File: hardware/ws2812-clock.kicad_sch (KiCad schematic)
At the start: 31 parts, among them J1 Conn_01x01_Pin, Q3 2N7002, SW2 Reset ESP, SW5 Toggle AP, SW6 Toggle Alarm, SW7 Snooze Alarm, U1 ESP32-WROOM-32D, U3 SHT30-DIS, U4 AMS1117-3.3, U5 DMP3026SFDE-7

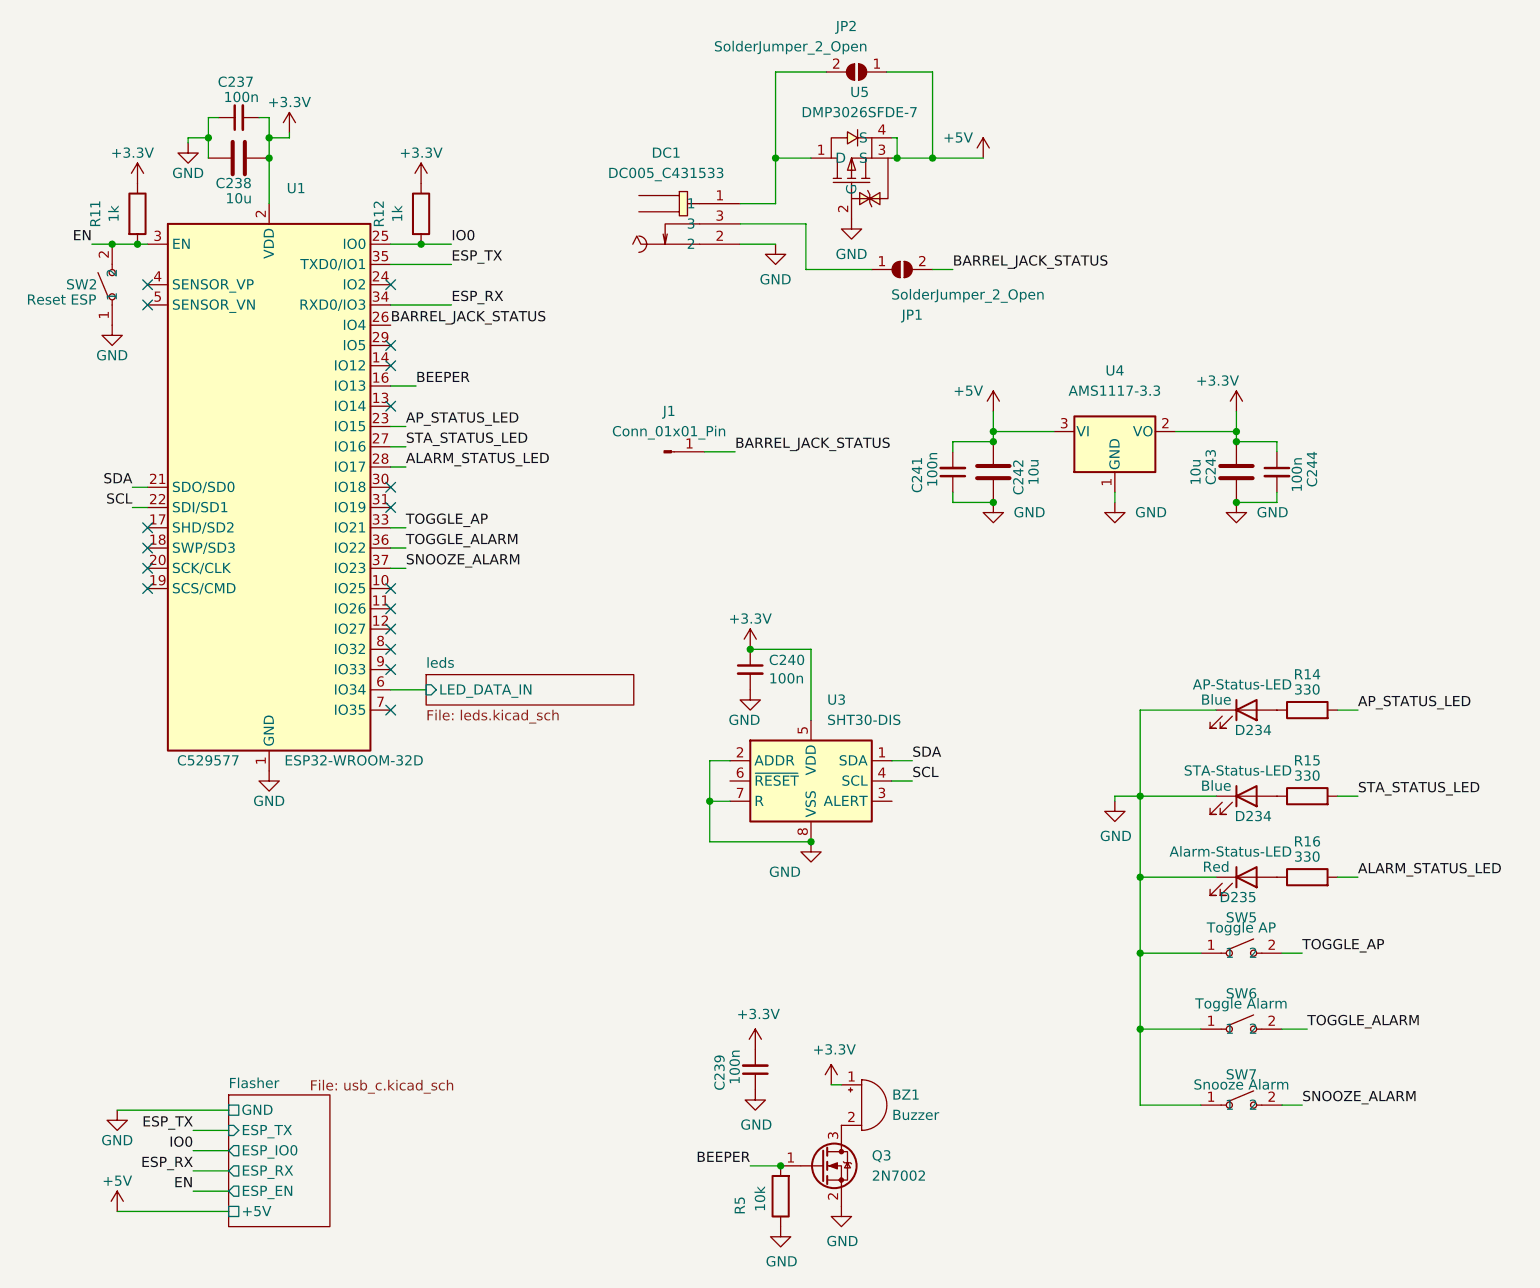
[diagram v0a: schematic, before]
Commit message: Updated PCB
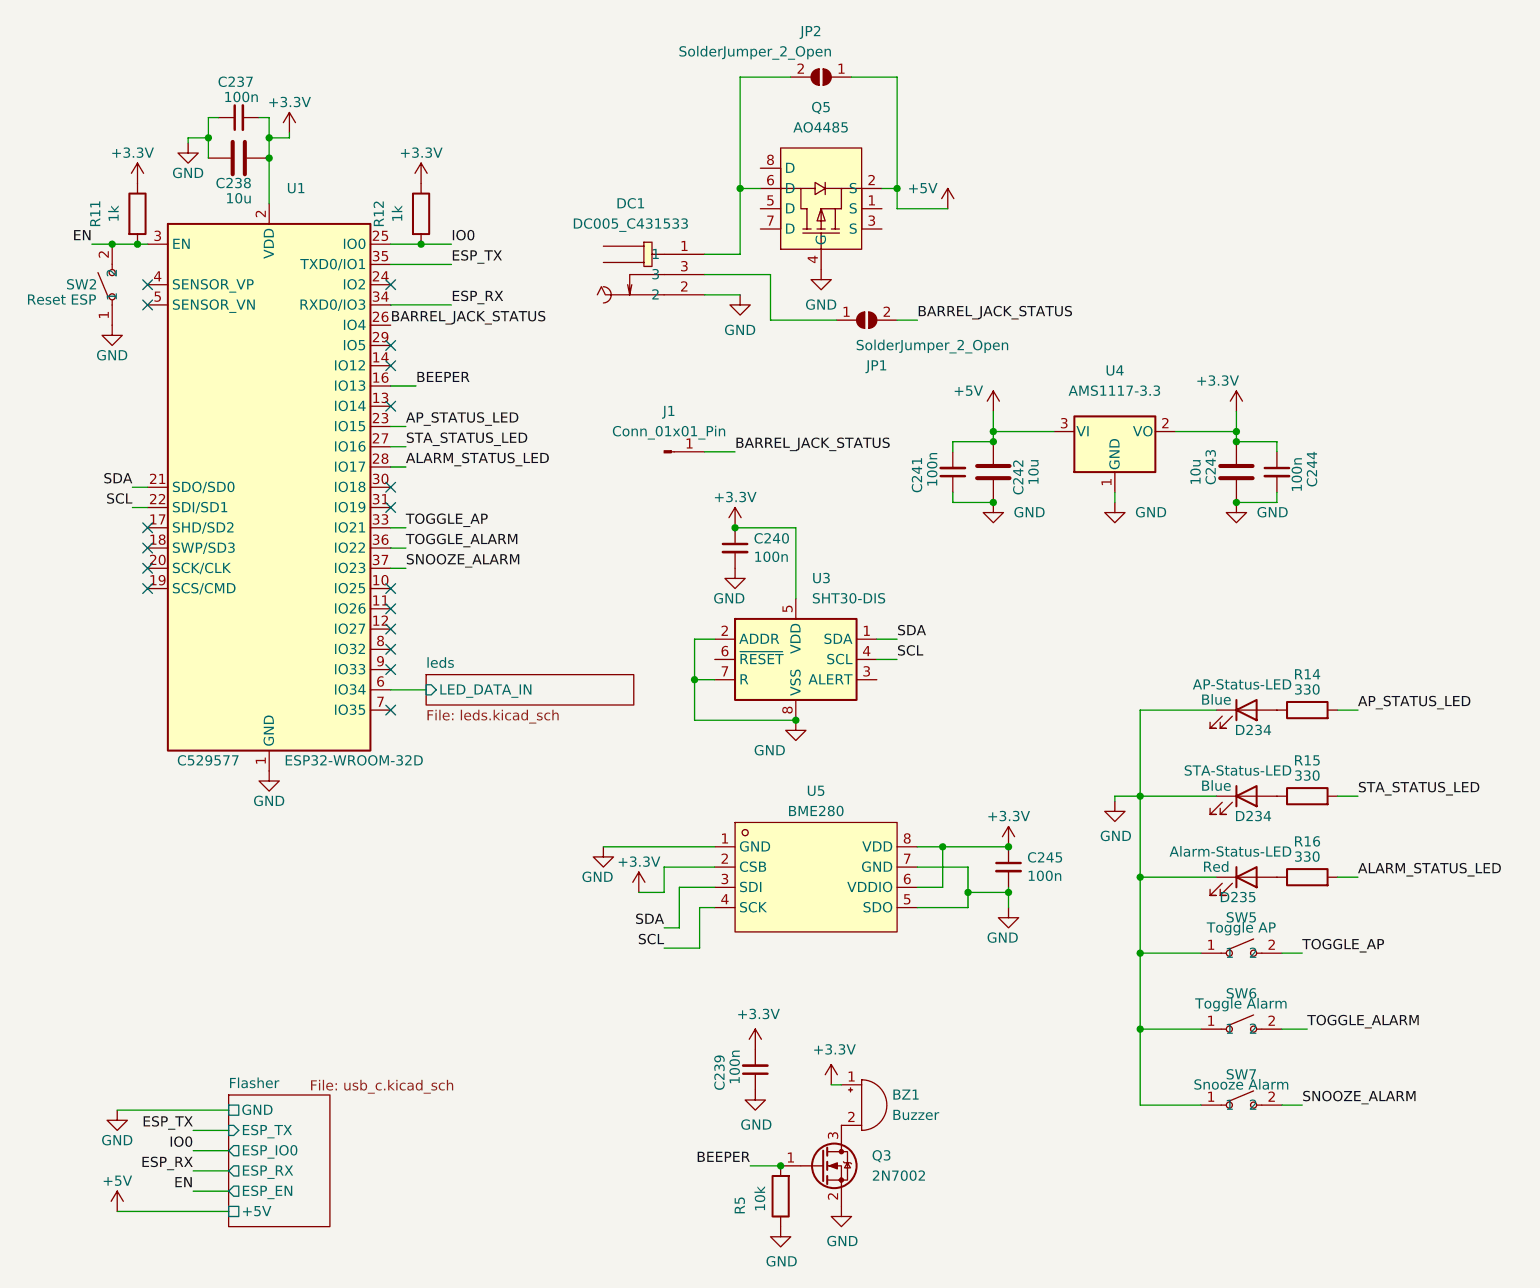
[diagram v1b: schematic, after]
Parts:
- removed U5: DMP3026SFDE-7, reverse_polarity_diode:U-DFN2020-6E_L2.0-W2.0-P0.65-BL, symbol reverse_polarity_diode:DMP3026SFDE-7
- added C245: 100n, Capacitor_SMD:C_0402_1005Metric, symbol Device:C_Small
- added Q5: AO4485, reverse_polarity_diode:SOIC-8_L5.0-W4.0-P1.27-LS6.0-BL, symbol reverse_polarity_diode:AO4485
- added U5: BME280, bme280:LGA-8_BME280_BL, symbol bme280:BME280
- J1: LCSC (none) -> DNP
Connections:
- net +3.3V: now also C245.1, U5.2 (CSB), U5.6 (VDDIO), U5.8 (VDD)
- net +5V: now also Q5.2 (S)
- net GND: now also C245.2, Q5.4 (G), U5.1 (GND), U5.5 (SDO), U5.7 (GND)
- net SCL: now also U5.4 (SCK)
- net SDA: now also U5.3 (SDI)
- net at DC1.1, JP2.2 (B): now also Q5.6 (D)
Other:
- moved on the sheet: C240, DC1, JP1, JP2, U3
